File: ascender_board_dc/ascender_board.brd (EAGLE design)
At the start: 94 x 82.8 mm, 125 parts, among them IC1 LM2937, IC2 MC33932, Q1 8MHz, Q2 BSS123, Q3 BSS123, Q4 BSS123, U1 STM32F722XX, U2 I2C EEPROM, X2 52745-1890, X3 52745-1890, X4 MINI-USB-SCHIELD-32005-201

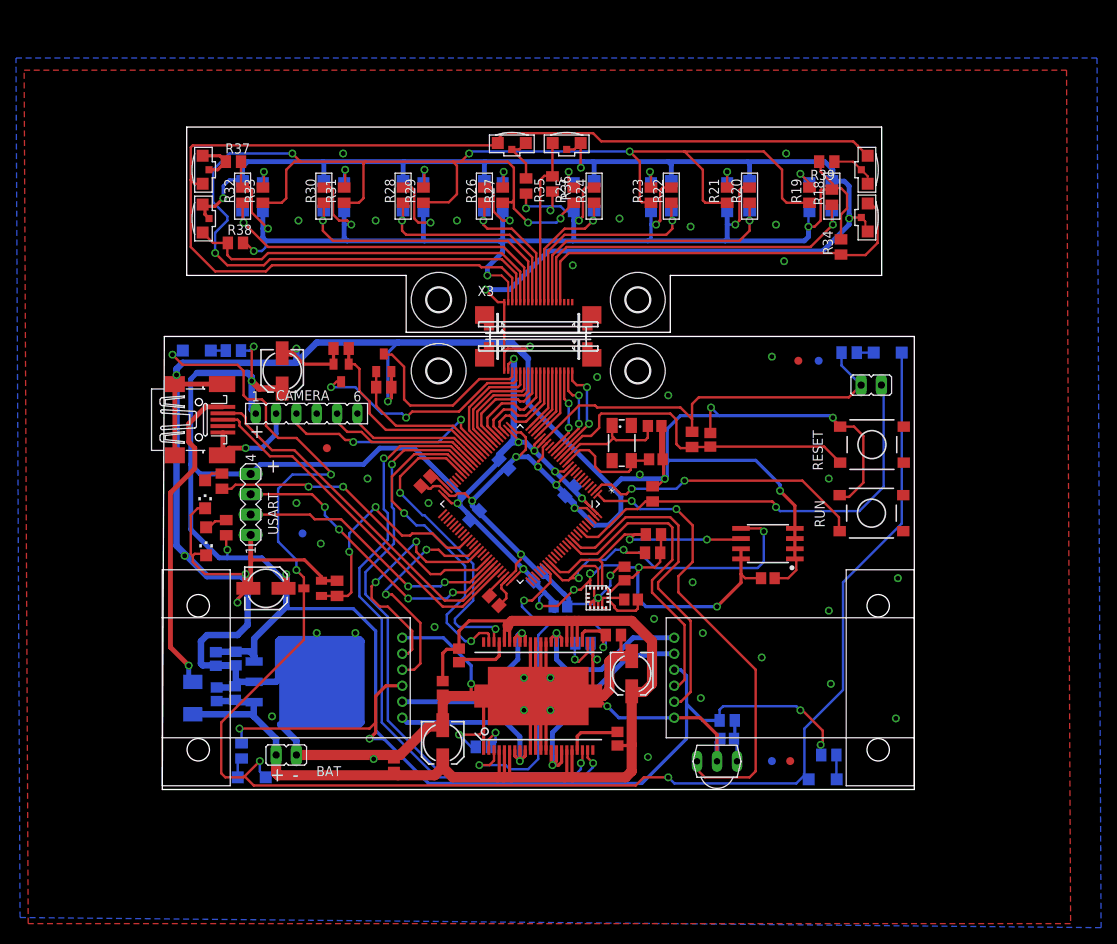
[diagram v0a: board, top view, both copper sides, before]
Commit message: board
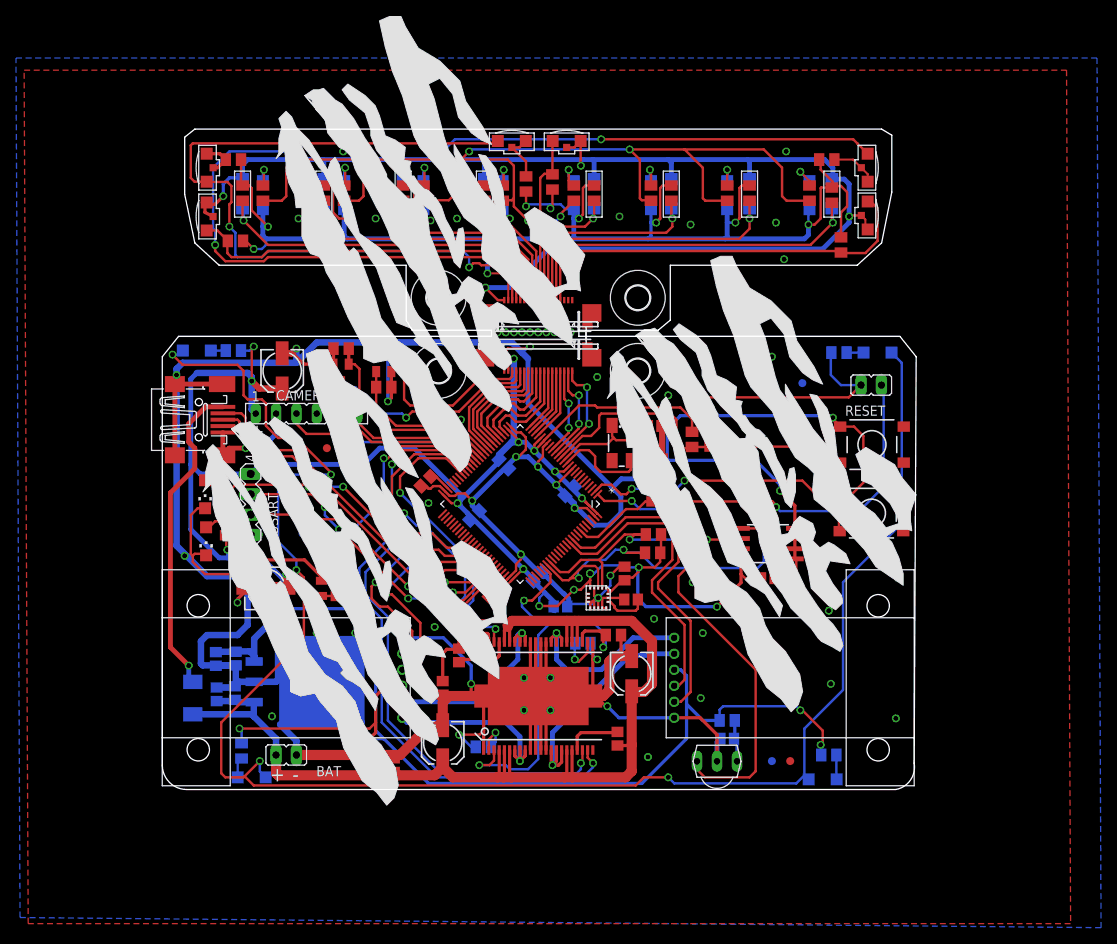
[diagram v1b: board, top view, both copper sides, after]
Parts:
- added U$21, U$22, U$24: (no value), shapes:SCAR
- added U$23, U$25: (no value), shapes:LIGHTNING
- moved U$8 3.45 mm to (80.0, 50.8)
- moved R14 1.27 mm to (84.6, 54.6)
- moved LED4 1.27 mm to (89.4, 54.6)
- moved U$30 0.57 mm to (6.35, 77.7)
- moved U$31 0.57 mm to (6.35, 71.6)
- moved H1 0.25 mm to (59.4, 61.5)
- moved H2 0.25 mm to (34.5, 61.5)
- moved LED10 0.25 mm to (51.4, 74.3)
- moved LED11 0.25 mm to (42.5, 74.3)
- moved LED12 0.25 mm to (32.6, 74.3)
- moved LED13 0.25 mm to (22.7, 74.3)
- moved LED14 0.25 mm to (12.6, 74.3)
- moved LED7 0.25 mm to (80.9, 74.3)
- moved LED8 0.25 mm to (70.6, 74.3)
- moved LED9 0.25 mm to (61.1, 74.3)
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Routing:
- net IR_B_S: track 146.4 -> 154.1 mm, vias 0 -> 4
- net GND: track 828.4 -> 823.0 mm, vias 66 -> 76
- net +3V3: track 632.8 -> 634.9 mm
- net IR_A_S: track 202.2 -> 200.8 mm
- net N$31: track 5.72 -> 4.70 mm
- net N$16: track 219.8 -> 220.3 mm
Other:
- board size 94 x 82.8 mm -> 94.2 x 82.5 mm
